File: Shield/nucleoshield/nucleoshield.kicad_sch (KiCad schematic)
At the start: 41 parts, among them IC1 L80-M39, J1 Conn_02x19_Odd_Even, J10 ENCODER_3, J11 MPU9250, J12 5V_DCDC, J13 3V3_DCDC, J2 Conn_02x19_Odd_Even, J3 Battery, J4 MOTOR_1, J5 ENCODER_1, J6 ENCODER_2, J7 MOTOR_2, J8 LCD_I2C, J9 MOTOR_3, Q1 BSS138, Q2 BSS138, Q3 AO3401A, Q4 AO3401A, Q5 AO3401A

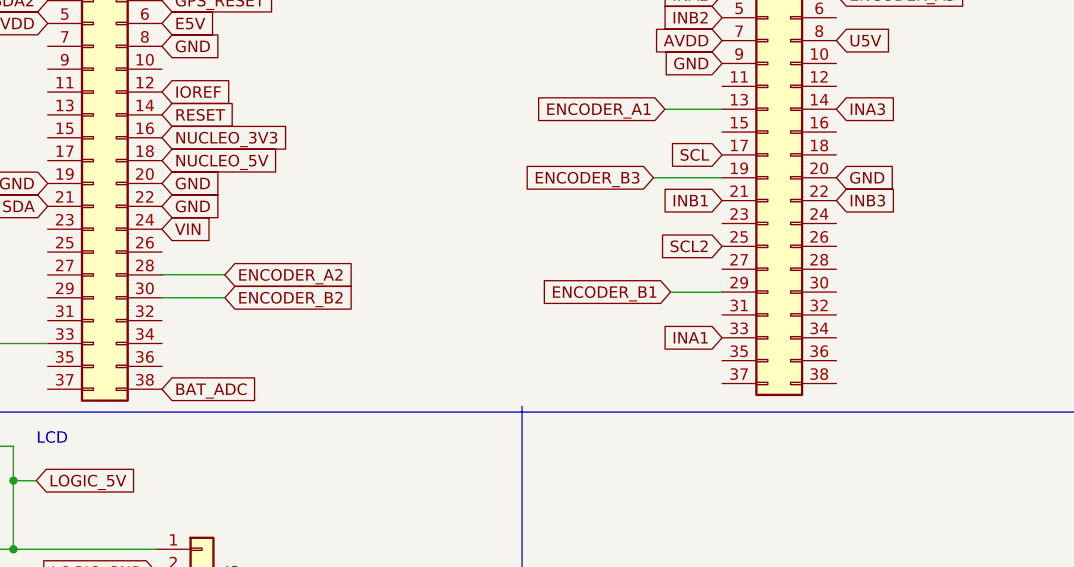
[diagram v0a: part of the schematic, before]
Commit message: Schematic update
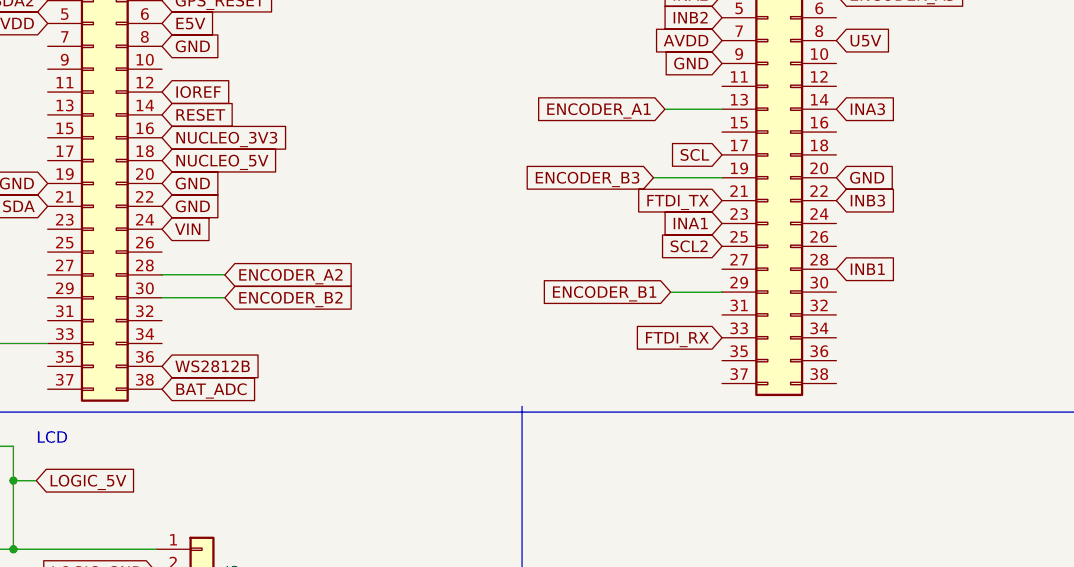
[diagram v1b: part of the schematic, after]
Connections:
- net INA1: now also J2.23 (Pin_23); no longer J2.33 (Pin_33)
- net INB1: now also J2.28 (Pin_28); no longer J2.21 (Pin_21)
- net WS2812B: now reaches J1.36 (Pin_36)
- new net FTDI_RX: J2.33 (Pin_33)
- new net FTDI_TX: J2.21 (Pin_21)
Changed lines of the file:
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@@
+    )
+  )
+  (global_label "WS2812B" (shape input) (at 132.715 115.57 0) (fields_autoplaced)
+    (effects (font (size 1.27 1.27)) (justify left))
+    (property "Intersheet References" "${INTERSHEET_REFS}" (id 0) (at 143.8971 115.6494 0)
+      (effects (font (size 1.27 1.27)) (justify left) hide)
     )
   )
@@
     )
   )
+  (global_label "FTDI_RX" (shape input) (at 194.945 112.395 180) (fields_autoplaced)
+    (effects (font (size 1.27 1.27)) (justify right))
+    (property "Intersheet References" "${INTERSHEET_REFS}" (id 0) (at 185.1538 112.3156 0)
+      (effects (font (size 1.27 1.27)) (justify right) hide)
+    )
+  )
   (global_label "3V3_DCDC" (shape input) (at 43.815 20.32 0) (fields_autoplaced)
     (effects (font (size 1.27 1.27)) (justify left))
@@
     )
   )
+  (global_label "FTDI_TX" (shape input) (at 194.945 97.155 180) (fields_autoplaced)
+    (effects (font (size 1.27 1.27)) (justify right))
+    (property "Intersheet References" "${INTERSHEET_REFS}" (id 0) (at 185.4562 97.0756 0)
+      (effects (font (size 1.27 1.27)) (justify right) hide)
+    )
+  )
   (global_label "RESET" (shape input) (at 132.715 87.63 0) (fields_autoplaced)
     (effects (font (size 1.27 1.27)) (justify left))
@@
     )
   )
-  (global_label "INA1" (shape input) (at 194.945 112.395 180) (fields_autoplaced)
-    (effects (font (size 1.27 1.27)) (justify right))
-    (property "Intersheet References" "${INTERSHEET_REFS}" (id 0) (at 188.2986 112.3156 0)
+  (global_label "INA1" (shape input) (at 194.945 99.695 180) (fields_autoplaced)
+    (effects (font (size 1.27 1.27)) (justify right))
+    (property "Intersheet References" "${INTERSHEET_REFS}" (id 0) (at 188.2986 99.6156 0)
       (effects (font (size 1.27 1.27)) (justify right) hide)
     )
@@
     )
   )
-  (global_label "INB1" (shape input) (at 194.945 97.155 180) (fields_autoplaced)
-    (effects (font (size 1.27 1.27)) (justify right))
-    (property "Intersheet References" "${INTERSHEET_REFS}" (id 0) (at 188.1171 97.0756 0)
-      (effects (font (size 1.27 1.27)) (justify right) hide)
-    )
-  )
+  (global_label "INB1" (shape input) (at 207.645 104.775 0) (fields_autoplaced)
+    (effects (font (size 1.27 1.27)) (justify left))
+    (property "Intersheet References" "${INTERSHEET_REFS}" (id 0) (at 214.4729 104.8544 0)
+      (effects (font (size 1.27 1.27)) (justify left) hide)
+    )
+  )
